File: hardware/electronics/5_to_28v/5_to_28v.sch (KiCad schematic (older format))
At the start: 29 parts

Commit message: add changesto arduino and hardware
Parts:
- A?: symbol MCU_Module:Arduino_Nano_v3.x -> 5_to_28v-rescue:Arduino_Nano_v3.x-MCU_Module
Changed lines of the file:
@@
 EESchema Schematic File Version 4
-LIBS:5_to_28v-cache
 EELAYER 30 0
 EELAYER END
@@
 	2100 4800 2300 4800
 $Comp
-L MCU_Module:Arduino_Nano_v3.x A?
+L 5_to_28v-rescue:Arduino_Nano_v3.x-MCU_Module A?
 U 1 1 5DCCC149
 P 2500 2500

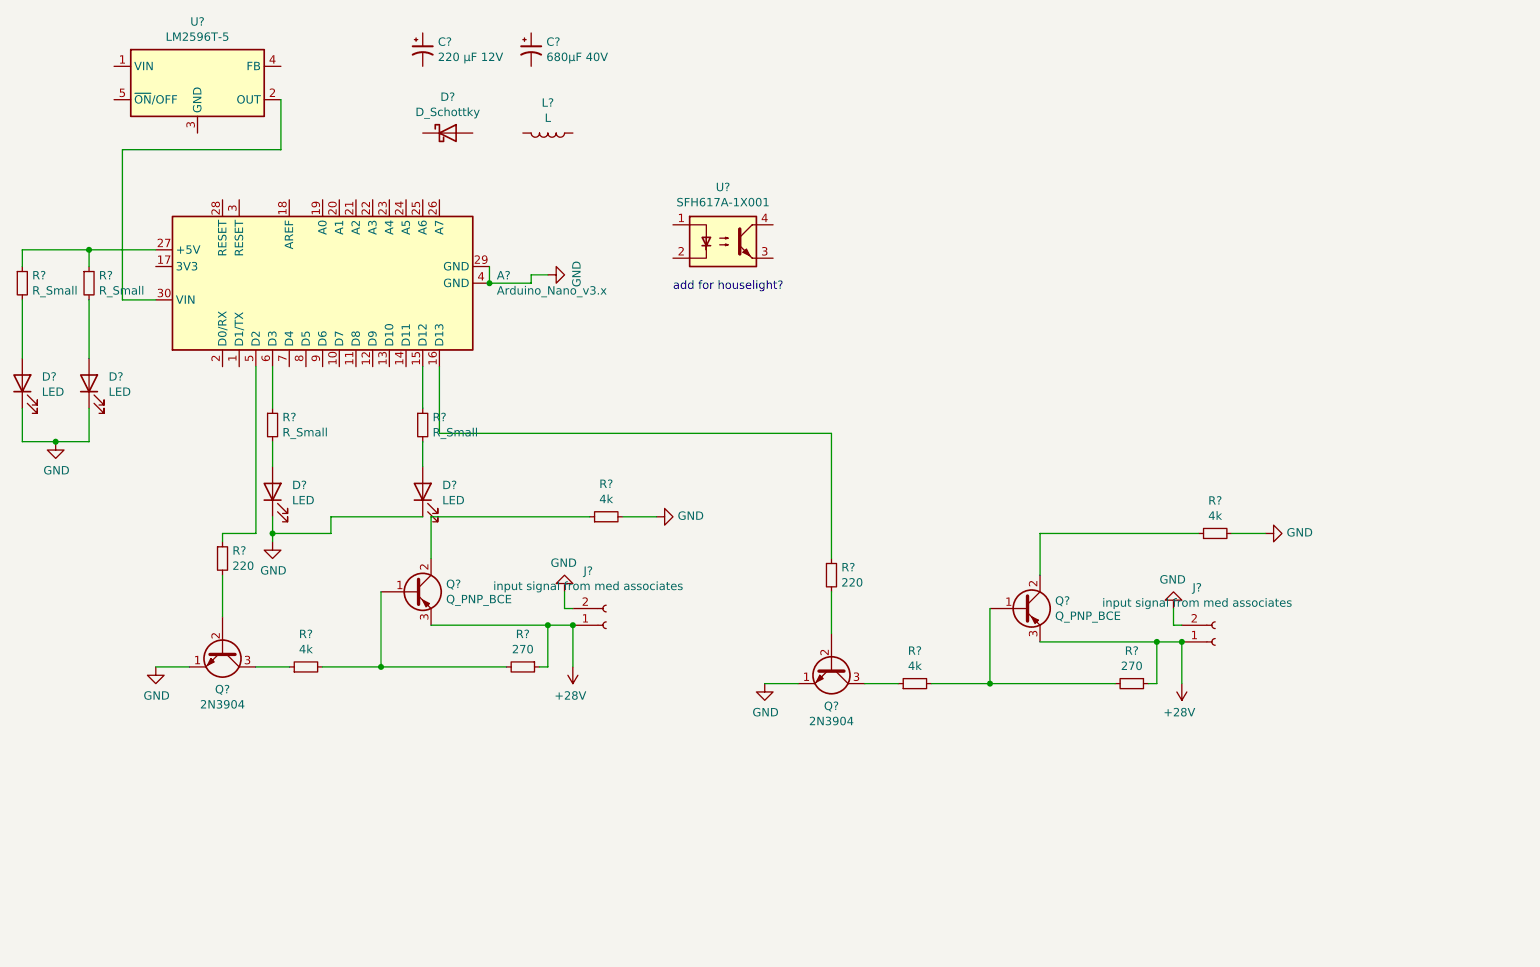
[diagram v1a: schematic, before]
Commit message: add baords and updates to code
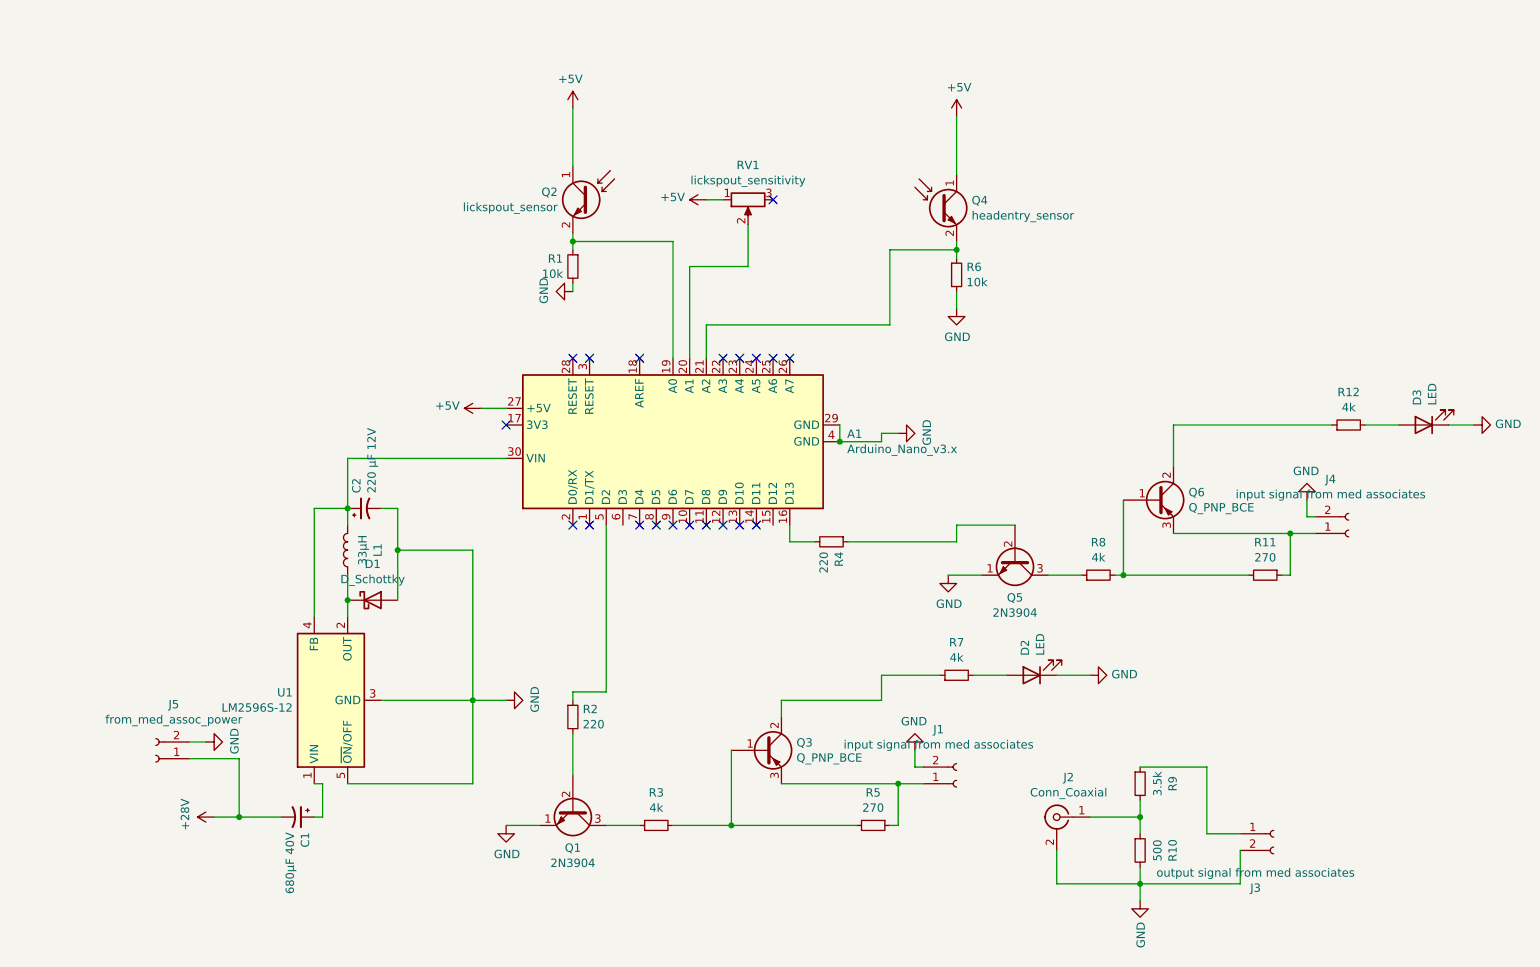
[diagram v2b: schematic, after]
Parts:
- removed D? (x4): LED, symbol Device:LED
- removed R? (x4): R_Small, symbol Device:R_Small
- removed U?: LM2596T-5, Package_TO_SOT_THT:TO-220-5_P3.4x3.7mm_StaggerOdd_Lead3.8mm_Vertical, symbol Regulator_Switching:LM2596T-5
- removed U?: SFH617A-1X001, Package_DIP:DIP-4_W7.62mm, symbol Isolator:SFH617A-1X001
- added D2, D3: LED, LED_THT:LED_D5.0mm, symbol Device:LED
- added J2: Conn_Coaxial, Connector_Coaxial:BNC_Amphenol_B6252HB-NPP3G-50_Horizontal, symbol Connector:Conn_Coaxial
- added J3: output signal from med associates, symbol Connector:Conn_01x02_Female
- added J5: from_med_assoc_power, symbol Connector:Conn_01x02_Female
- added Q2: lickspout_sensor, LED_THT:LED_D5.0mm, symbol Device:Q_Photo_NPN
- added Q4: headentry_sensor, LED_THT:LED_D5.0mm, symbol Device:Q_Photo_NPN
- added R1, R6: 10k, symbol Device:R_Small
- added R10: 500, symbol Device:R_Small
- added R9: 3.5k, symbol Device:R_Small
- added RV1: lickspout_sensitivity, Potentiometer_THT:Potentiometer_ACP_CA6-H2,5_Horizontal, symbol Device:R_POT
- added U1: LM2596S-12, Package_TO_SOT_SMD:TO-263-5_TabPin3, symbol Regulator_Switching:LM2596S-12
- C1, C2: renamed from C?; footprint (none) -> Capacitor_THT:CP_Radial_D10.0mm_P5.00mm_P7.50mm
- D1: renamed from D?; footprint (none) -> Diode_THT:D_DO-27_P15.24mm_Horizontal
- L1: renamed from L?; value L -> 33µH
- gave numbers to parts that had none: 15
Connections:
- net +28V: now also C1.2, J5.1 (Pin_1); no longer J1.1 (Pin_1), J4.1 (Pin_1), Q3.3 (E), Q6.3 (E), R11.1, R5.1
- net GND: now also C2.2, D1.2 (A), D2.1 (K), D3.1 (K), J2.2 (Ext), J3.2 (Pin_2), J5.2 (Pin_2), R1.2, R10.2, R6.2, U1.3 (GND), U1.5 (~ON~/OFF); no longer R12.2, R7.2
- net at A1.16 (D13): now also R4.2; no longer R4.1
- net at A1.19 (A0): now also Q2.2 (E), R1.1
- net at A1.20 (A1): now also RV1.2
- net at A1.21 (A2): now also Q4.2 (E), R6.1
- net +5V: now reaches A1.27 (+5V)
- net +5V: now also Q2.1 (C), Q4.1 (C), RV1.1
- net at A1.30 (VIN): now also C2.1, L1.2, U1.4 (FB)
- net at C1.1: now also U1.1 (VIN)
- net at D1.1 (K): now also L1.1, U1.2 (OUT)
- net at Q5.2 (B): now also R4.1; no longer R4.2
- new net: J1.1 (Pin_1), Q3.3 (E), R5.1
- new net: D2.2 (A), R7.2
- new net: D3.2 (A), R12.2
- new net: J4.1 (Pin_1), Q6.3 (E), R11.1
- new net: J3.1 (Pin_1), R9.1
- new net: J2.1 (In), R10.1, R9.2
- no-connect marks 0 -> 20
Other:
- note removed: "add for houselight?\n"
- moved on the sheet: A1, C1, C2, D1, J1, J4, L1, Q1, Q3, Q5, Q6, R11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
